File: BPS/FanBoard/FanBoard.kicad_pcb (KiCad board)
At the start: 2 copper layers, 36.2 x 26 mm, 19 parts, among them J1 Conn_01x02, J2 Conn_01x02, J3 Conn_01x02, J4 Conn_01x02, J5 LDRBRDConn, Q1 BUK9M34-100EX, Q2 BUK9M34-100EX, Q3 BUK9M34-100EX, Q4 BUK9M34-100EX

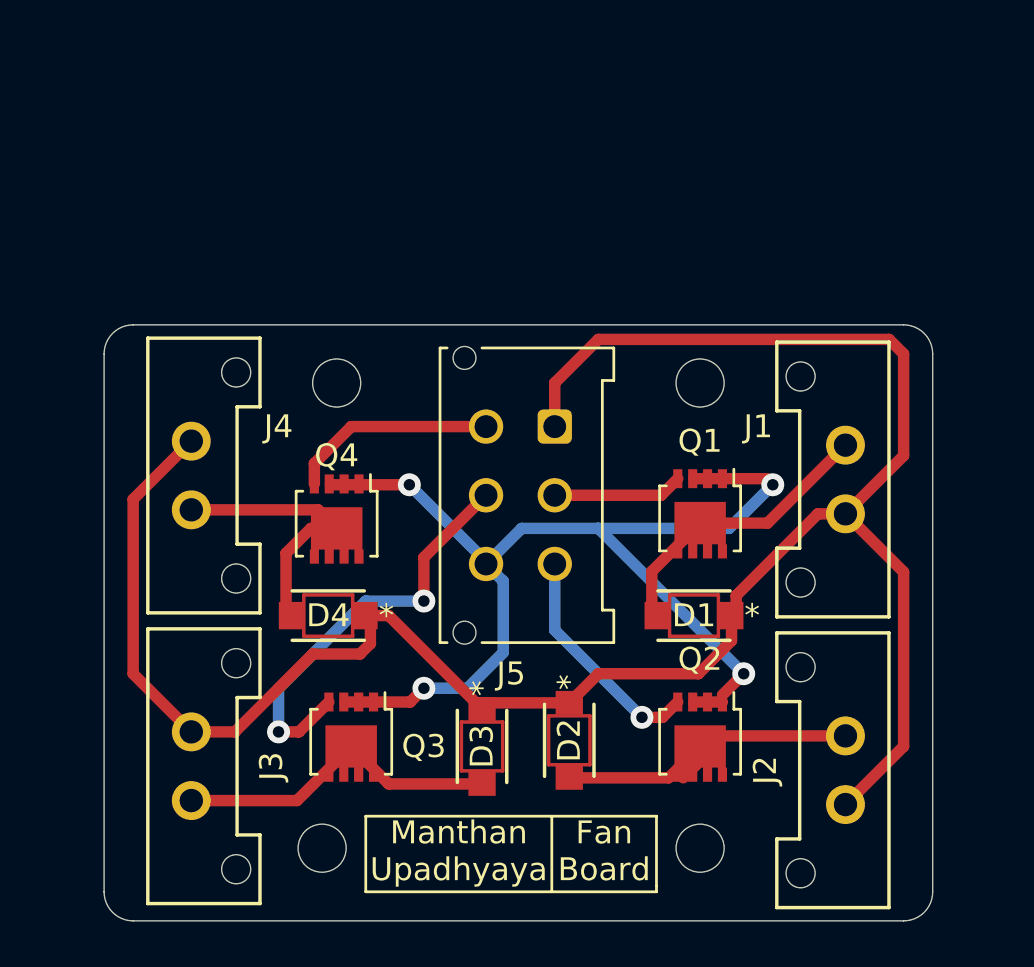
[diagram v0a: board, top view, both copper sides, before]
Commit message: Redid layout of board
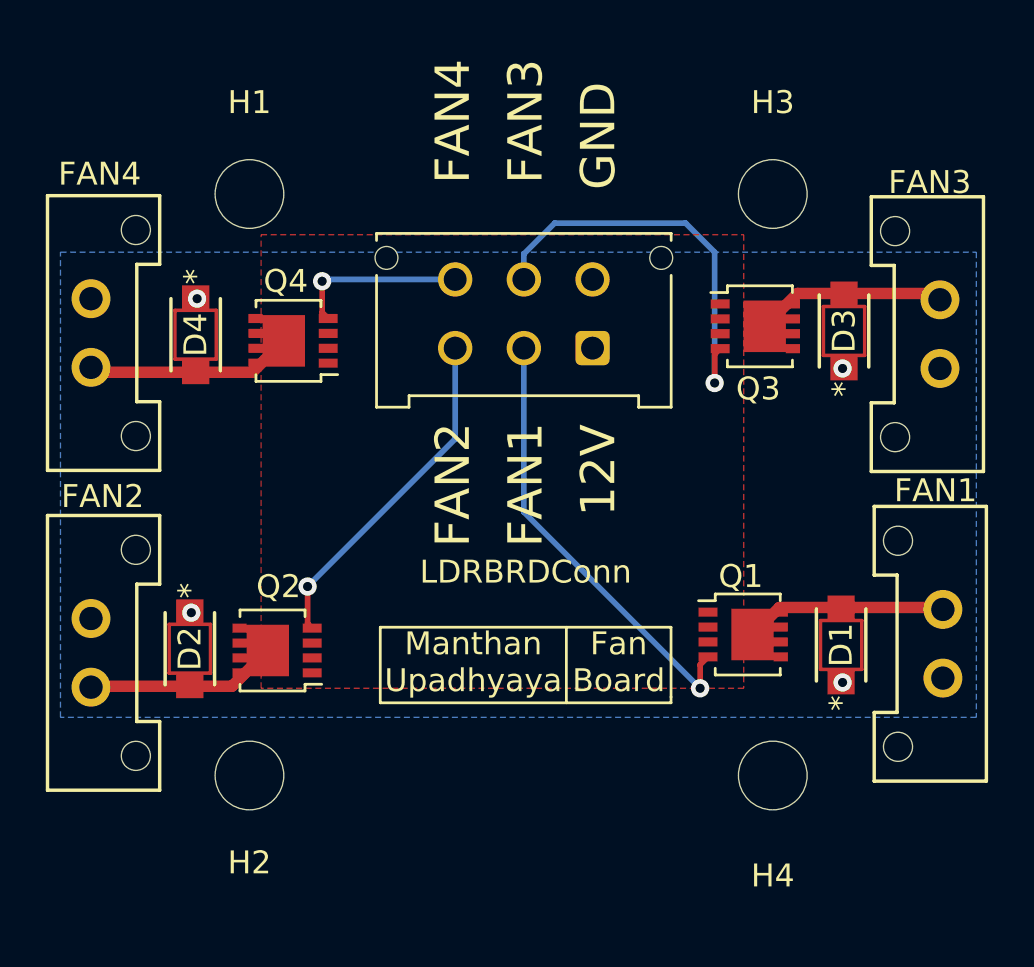
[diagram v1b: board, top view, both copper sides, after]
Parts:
- removed G***: LOGO, UTSVT_Special:Hallock_Image_Small
- removed G***: LOGO, UTSVT_Special:UTSVT_Logo_Symbol
- removed J1: Conn_01x02, UTSVT_Connectors:Molex_MicroFit3.0_1x2xP3.00mm_PolarizingPeg_Vertical
- removed J5: LDRBRDConn, Connector_Molex:Molex_Micro-Fit_3.0_43045-0612_2x03_P3.00mm_Vertical
- removed REF** (x4): MountingHole_2.1mm, MountingHole:MountingHole_2.1mm
- added FAN1: Conn_01x02, UTSVT_Connectors:Molex_MicroFit3.0_1x2xP3.00mm_PolarizingPeg_Vertical, F.Cu at (176.3, 80.8)
- added H1: MountingHole, MountingHole:MountingHole_3mm, F.Cu at (146.1, 59.7)
- added H2: MountingHole, MountingHole:MountingHole_3mm, F.Cu at (146.1, 85.1)
- added H3: MountingHole, MountingHole:MountingHole_3mm, F.Cu at (168.9, 59.7)
- added H4: MountingHole, MountingHole:MountingHole_3mm, F.Cu at (168.9, 85.1)
- added LDRBRDConn: LDRBRDConn, Connector_Molex:Molex_Micro-Fit_3.0_43045-0612_2x03_P3.00mm_Vertical, F.Cu at (161.0, 66.4)
- moved FAN3 36.4 mm to (176.2, 67.3), turned to 90 degrees
- moved FAN2 33.9 mm to (139.1, 78.2), turned to 270 degrees
- moved Q3 25.2 mm to (168.1, 65.5), turned to 0 degrees
- moved D3 24.1 mm to (172.0, 65.7), turned to 90 degrees
- moved Q2 18.9 mm to (147.3, 79.6), turned to 180 degrees
- moved D2 17.0 mm to (143.4, 79.6)
- moved D4 13.6 mm to (143.7, 65.8), turned to 270 degrees
- moved Q4 8.02 mm to (148.0, 66.1), turned to 180 degrees
- moved FAN4 7.61 mm to (139.1, 64.3)
- moved D1 6.55 mm to (171.9, 79.4), turned to 90 degrees
- moved Q1 5.60 mm to (167.6, 78.9), turned to 0 degrees
- renumbered J2 to FAN2, J3 to FAN3, J4 to FAN4
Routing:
- net +12V: track 93.6 -> 0.00 mm, vias 0 -> 4
- net GNDPWR: track 49.4 -> 0.00 mm, vias 4 -> 0
- net /FAN1: track 5.68 -> 19.6 mm, vias 0 -> 1
- net Net-(D3-Pad2): track 14.4 -> 8.37 mm
- net Net-(D2-Pad2): track 13.9 -> 8.39 mm
- net /FAN2: track 10.2 -> 15.0 mm
- net Net-(D1-Pad2): track 12.7 -> 8.84 mm
- net Net-(D4-Pad2): track 12.1 -> 9.08 mm
- net /FAN4: track 9.06 -> 7.58 mm, vias 0 -> 1
- net /FAN3: track 18.3 -> 17.8 mm, vias 2 -> 1
- added copper zone on B.Cu, net +12V
- added copper zone on F.Cu, net GNDPWR
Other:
- board outline removed
- board text added: "12V"
- board text added: "FAN1"
- board text added: "FAN2"
- board text added: "FAN3"
- board text added: "FAN4"
- board text added: "GND"
